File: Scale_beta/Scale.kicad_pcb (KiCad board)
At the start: 2 copper layers, 128.4 x 60 mm, 16 parts, among them J1 Conn_01x04_Female, J2 Conn_01x03_Female, J3 Conn_01x07_Female, J4 Conn_01x07_Female, J5 Conn_01x07_Male

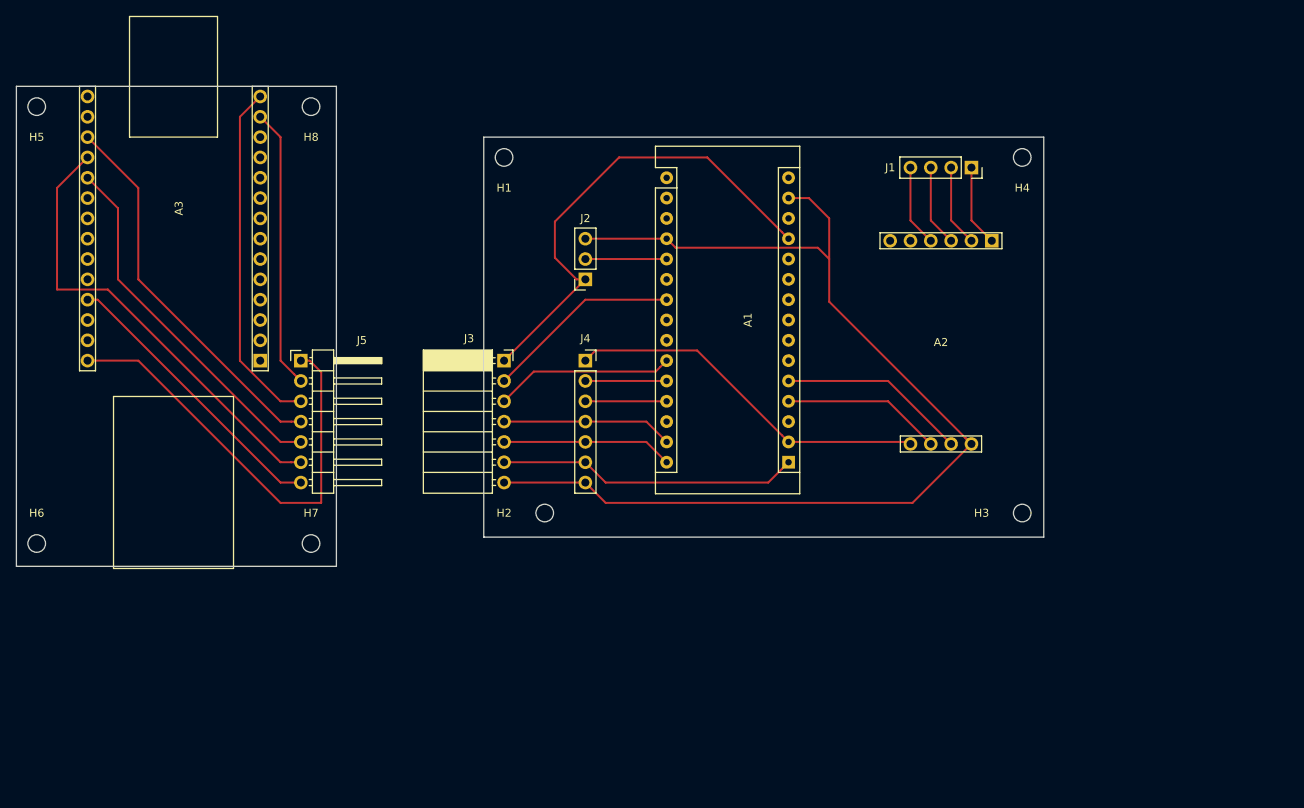
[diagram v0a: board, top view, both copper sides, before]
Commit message: Beta version
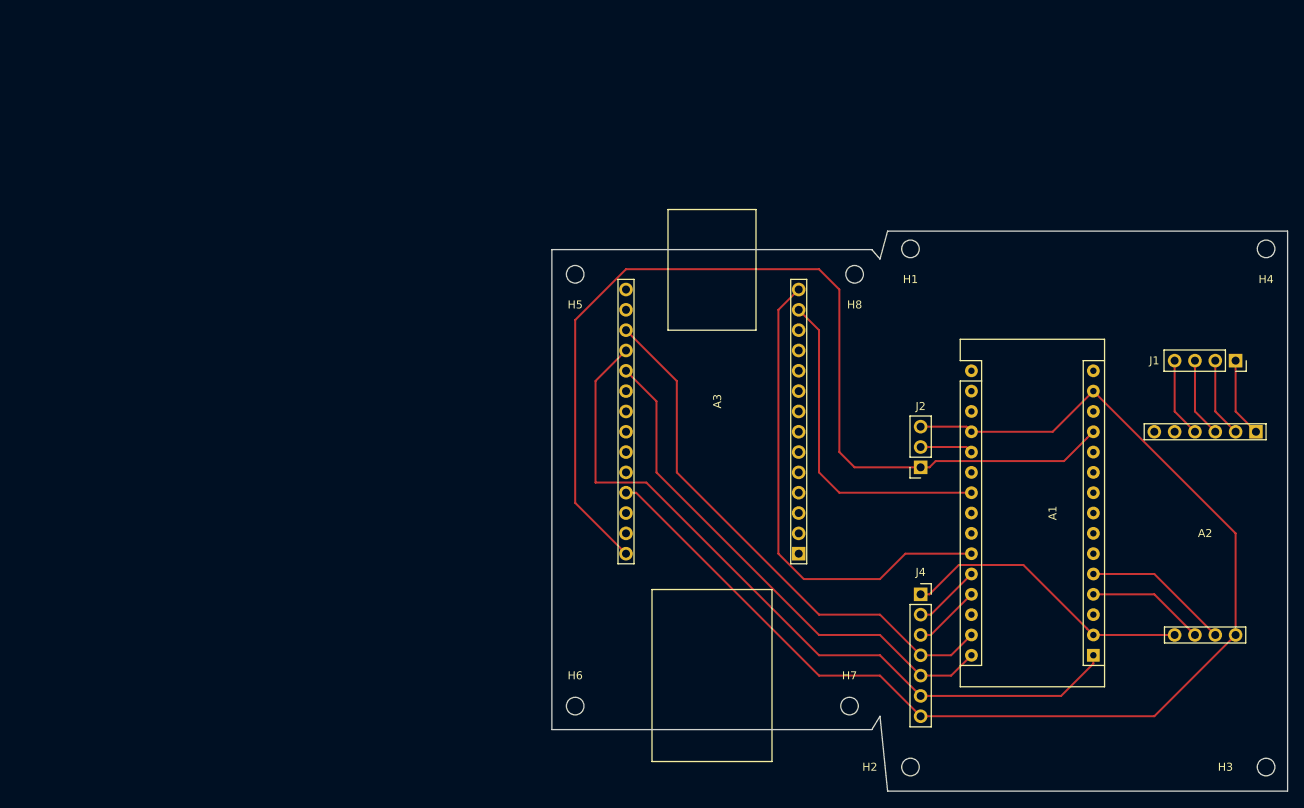
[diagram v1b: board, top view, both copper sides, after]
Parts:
- removed J3: Conn_01x07_Female, Connector_PinSocket_2.54mm:PinSocket_1x07_P2.54mm_Horizontal
- removed J5: Conn_01x07_Male, Connector_PinHeader_2.54mm:PinHeader_1x07_P2.54mm_Horizontal
- moved A3 71.5 mm to (141.0, 104.1)
- moved H8 71.1 mm to (148.0, 69.2)
- moved H5 70.5 mm to (113.0, 69.2)
- moved H6 70.3 mm to (113.0, 123.2)
- moved H7 70.3 mm to (147.3, 123.2)
- moved H2 55.7 mm to (154.9, 130.8)
- moved H1 52.1 mm to (154.9, 66.0)
- moved J4 51.1 mm to (156.2, 109.2)
- moved J2 48.0 mm to (156.2, 93.3)
- moved A1 45.1 mm to (177.8, 116.8)
- moved H3 44.0 mm to (199.4, 130.8)
- moved J1 40.9 mm to (195.6, 80.0)
- moved A2 40.7 mm to (185.4, 88.9)
- moved H4 32.6 mm to (199.4, 66.0)
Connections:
- net S renamed RELAY
- A3 pad 13: Net-(A3-Pad13) -> SS_SD
- A3 pad 14: Net-(A3-Pad14) -> SS_ETH
- A3 pad 17: Net-(A3-Pad17) -> MOSI
- A3 pad 18: Net-(A3-Pad18) -> SCK
- A3 pad 19: Net-(A3-Pad19) -> MISO
- A3 pad 25: Net-(A3-Pad25) -> GND
- A3 pad 28: Net-(A3-Pad28) -> +5V
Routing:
- net +5V: track 60.6 -> 123.2 mm
- net Net-(A3-Pad18): track 57.5 -> 0.00 mm
- net SCK: track 37.7 -> 94.1 mm
- net Net-(A3-Pad28): track 56.1 -> 0.00 mm
- net Net-(A3-Pad17): track 48.1 -> 0.00 mm
- net MOSI: track 21.4 -> 67.8 mm
- net Net-(A3-Pad19): track 45.6 -> 0.00 mm
- net MISO: track 21.4 -> 65.2 mm
- net Net-(A3-Pad14): track 43.8 -> 0.00 mm
- net SS_ETH: track 22.4 -> 60.8 mm
- net Net-(A3-Pad25): track 36.1 -> 0.00 mm
- net Net-(A3-Pad13): track 35.1 -> 0.00 mm
- net SS_SD: track 24.5 -> 41.5 mm
- net GND: track 136.9 -> 153.8 mm
- net +3V3: track 46.0 -> 36.9 mm
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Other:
- board size 128.4 x 60 mm -> 92 x 70 mm
